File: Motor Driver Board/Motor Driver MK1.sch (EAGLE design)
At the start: 82 parts, among them IC1 REG1117

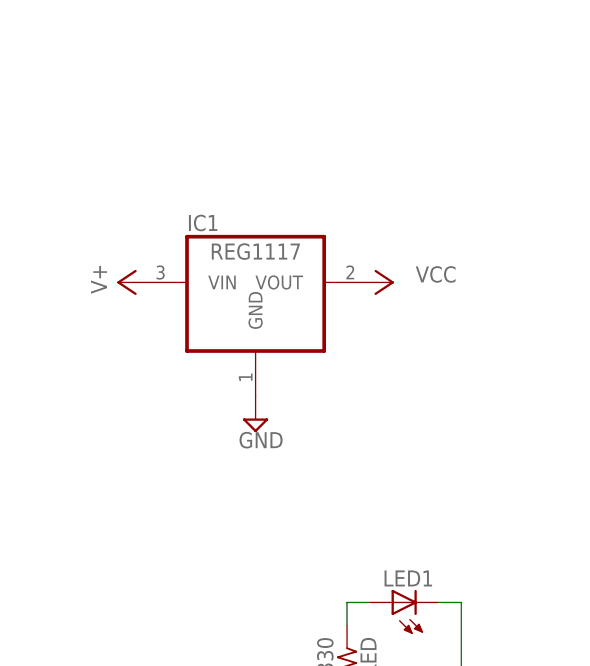
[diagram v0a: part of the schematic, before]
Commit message: Day 2. Everything is lines. How much further can this go?
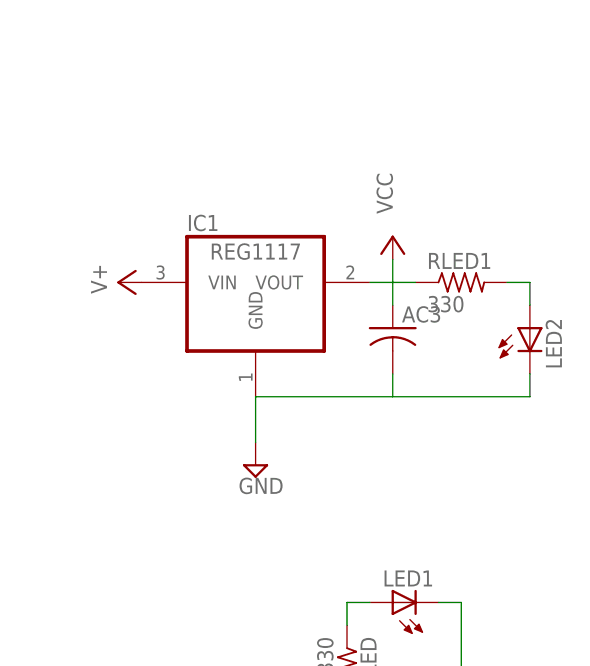
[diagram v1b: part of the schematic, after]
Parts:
- added AC3: (no value), rcl:C-USC0805
- added LED2: (no value), led:LEDCHIP-LED0805
- added RLED1: 330, resistor:R-US_R0805
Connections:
- new net N$31: LED2.A, RLED1.2
- net GND: now also AC3.2, LED2.C
- net VCC: now also AC3.1, RLED1.1
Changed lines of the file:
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@@
 <part name="P+23" library="supply1" deviceset="VCC" device=""/>
 <part name="P+24" library="supply1" deviceset="VCC" device=""/>
+<part name="AC3" library="rcl" deviceset="C-US" device="C0805"/>
+<part name="RLED1" library="resistor" deviceset="R-US_" device="R0805" value="330"/>
+<part name="LED2" library="led" deviceset="LED" device="CHIP-LED0805"/>
 </parts>
 <sheets>
@@
 <instance part="IC1" gate="G$1" x="220.98" y="137.16"/>
 <instance part="SUPPLY49" gate="1" x="205.74" y="137.16" rot="R90"/>
-<instance part="SUPPLY50" gate="GND" x="220.98" y="121.92"/>
-<instance part="P+19" gate="VCC" x="236.22" y="137.16" smashed="yes" rot="R270">
-<attribute name="VALUE" x="238.76" y="137.16" size="1.778" layer="96"/>
+<instance part="SUPPLY50" gate="GND" x="220.98" y="116.84"/>
+<instance part="P+19" gate="VCC" x="236.22" y="142.24" smashed="yes">
+<attribute name="VALUE" x="236.22" y="144.78" size="1.778" layer="96" rot="R90"/>
 </instance>
 <instance part="P+20" gate="VCC" x="165.1" y="152.4" smashed="yes">
@@
 <attribute name="VALUE" x="165.1" y="-22.86" size="1.778" layer="96" rot="R90"/>
 </instance>
+<instance part="AC3" gate="G$1" x="236.22" y="132.08"/>
+<instance part="RLED1" gate="G$1" x="243.84" y="137.16"/>
+<instance part="LED2" gate="G$1" x="251.46" y="132.08"/>
 </instances>
 <busses>
@@
 <pinref part="IC1" gate="G$1" pin="GND"/>
 <pinref part="SUPPLY50" gate="GND" pin="GND"/>
+<wire x1="220.98" y1="119.38" x2="220.98" y2="124.46" width="0.1524" layer="91"/>
+<pinref part="LED2" gate="G$1" pin="C"/>
+<wire x1="251.46" y1="127" x2="251.46" y2="124.46" width="0.1524" layer="91"/>
+<pinref part="AC3" gate="G$1" pin="2"/>
+<wire x1="251.46" y1="124.46" x2="236.22" y2="124.46" width="0.1524" layer="91"/>
+<wire x1="236.22" y1="127" x2="236.22" y2="124.46" width="0.1524" layer="91"/>
+<wire x1="236.22" y1="124.46" x2="220.98" y2="124.46" width="0.1524" layer="91"/>
 </segment>
 </net>
@@
 <pinref part="IC1" gate="G$1" pin="VOUT"/>
 <pinref part="P+19" gate="VCC" pin="VCC"/>
+<wire x1="236.22" y1="139.7" x2="236.22" y2="137.16" width="0.1524" layer="91"/>
+<pinref part="AC3" gate="G$1" pin="1"/>
+<wire x1="236.22" y1="137.16" x2="233.68" y2="137.16" width="0.1524" layer="91"/>
+<wire x1="236.22" y1="134.62" x2="236.22" y2="137.16" width="0.1524" layer="91"/>
+<pinref part="RLED1" gate="G$1" pin="1"/>
+<wire x1="236.22" y1="137.16" x2="238.76" y2="137.16" width="0.1524" layer="91"/>
 </segment>
 <segment>
@@
 </segment>
 </net>
+<net name="N$31" class="0">
+<segment>
+<pinref part="RLED1" gate="G$1" pin="2"/>
+<pinref part="LED2" gate="G$1" pin="A"/>
+<wire x1="248.92" y1="137.16" x2="251.46" y2="137.16" width="0.1524" layer="91"/>
+<wire x1="251.46" y1="137.16" x2="251.46" y2="134.62" width="0.1524" layer="91"/>
+</segment>
+</net>
